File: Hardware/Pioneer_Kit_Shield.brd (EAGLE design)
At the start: 53.3 x 59.7 mm, 38 parts, among them U1 USD-SOCKETNEW, U2 ARDUINO_UNO_R3_SHIELDNOLABELS, U3 HEX_CONVERTER, U4 PCA9306, U5 3.3V

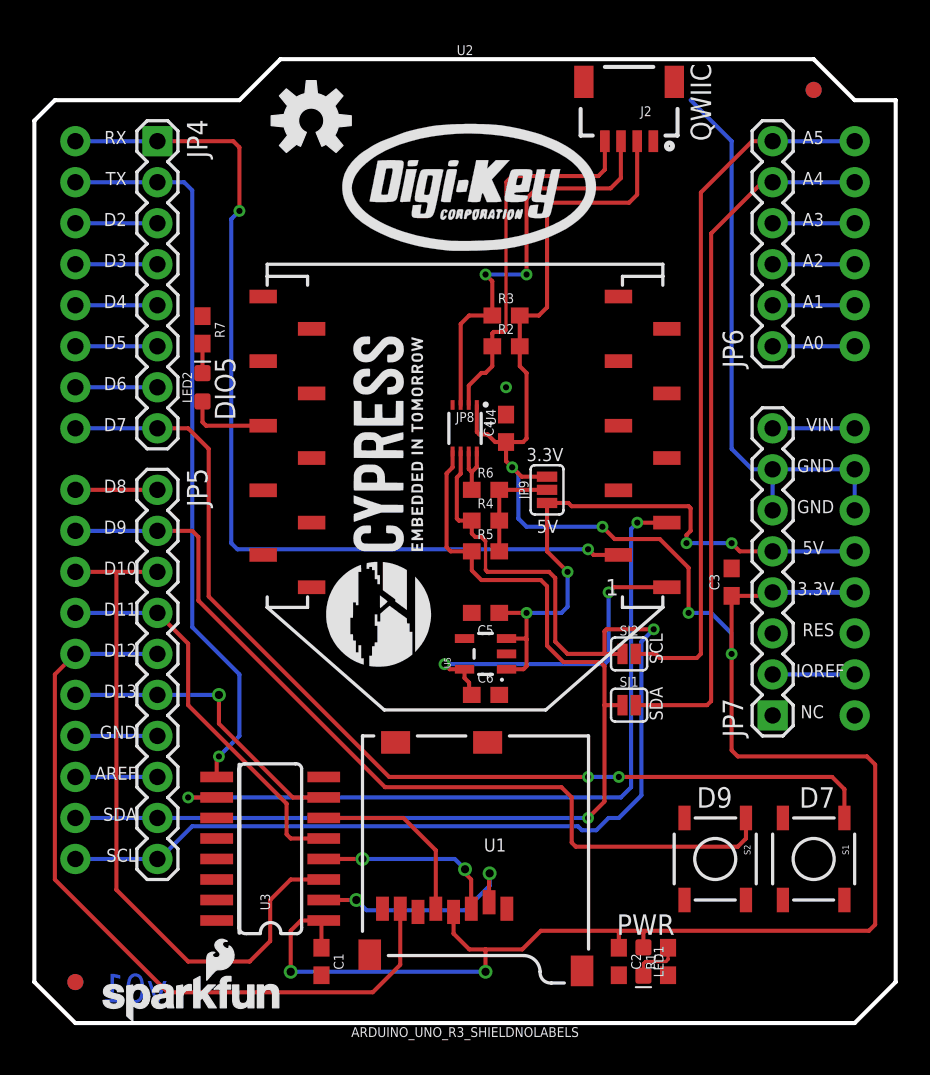
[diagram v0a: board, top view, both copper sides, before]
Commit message: Final version before review
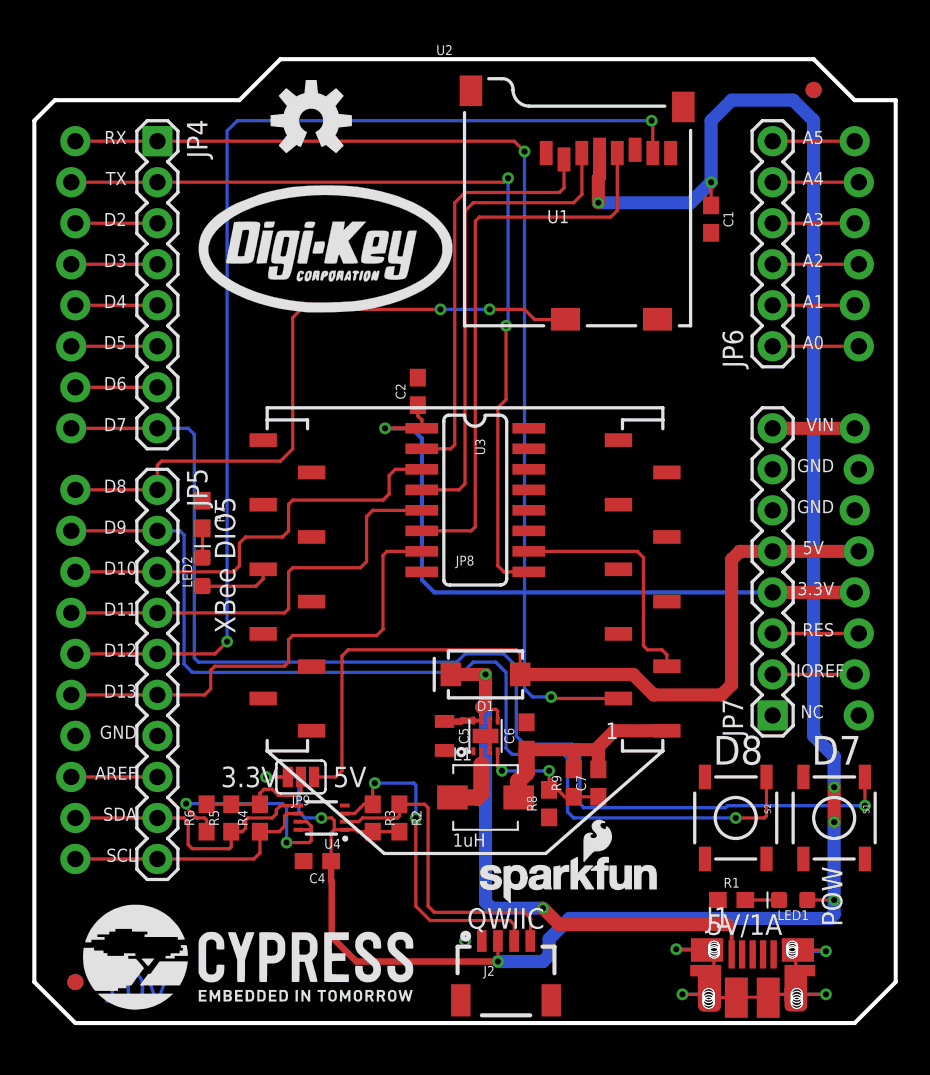
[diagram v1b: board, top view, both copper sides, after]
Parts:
- removed C3: 10uF, SparkFun-Capacitors:0603
- removed SJ1, SJ2: JUMPER-SMT_2_NC_PASTE_SILK, SparkFun-Jumpers:SMT-JUMPER_2_NC_PASTE_SILK
- added C7: 22pF, SparkFun-Capacitors:0603
- added D1: 3A/40V/500mV, SparkFun-DiscreteSemi:SMA-DIODE
- added FRAME2: FRAME-LETTERNO_PACKAGE, SparkFun-Aesthetics:DUMMY
- added J1: AMP FCI 10103594-0001LF, SparkFun-Connectors:USB-MICROB-PTH
- added L1: 1uH, SparkFun-Coils:INDUCTOR-SRP4020
- added R8: 180k, SparkFun-Resistors:0603
- added R9: 820k, SparkFun-Resistors:0603
- C5: value 1.0uF -> 10uF; device SparkFun-Capacitors:0603 -> SparkFun-Capacitors:0805
- C6: value 1.0uF -> 10uF
- U2: value ARDUINO_UNO_R3_SHIELDNOLABELS -> ARDUINO_UNO_R3_SHIELDUNO_R3_SHIELD_NOLABELS_LOCK; device SparkFun-Boards:UNO_R3_SHIELD_NOLABELS -> SparkFun-Boards:UNO_R3_SHIELD_NOLABELS_LOCK
- U5: value 3.3V -> TPS62065; device SparkFun-IC-Power:SOT23-5 -> SparkFun-IC-Power:WSON-8-PAD
- moved C1 51.9 mm to (40.6, 49.8)
- moved J2 50.1 mm to (27.9, 5.08), turned to 0 degrees
- moved C2 37.4 mm to (22.5, 39.1), turned to 90 degrees
- moved U1 32.5 mm to (39.4, 43.2), turned to 0 degrees
- moved R3 32.2 mm to (19.7, 12.7), turned to 270 degrees
- moved R2 29.9 mm to (21.3, 12.7), turned to 270 degrees
- moved C4 29.2 mm to (16.3, 10.0), turned to 180 degrees
- moved R6 26.7 mm to (9.40, 12.7), turned to 90 degrees
- moved U4 25.7 mm to (16.5, 12.7), turned to 90 degrees
- moved U3 25.0 mm to (26.0, 32.4), turned to 270 degrees
- moved JP1 24.5 mm to (25.9, 7.37)
- moved JP9 23.4 mm to (15.2, 15.2), turned to 180 degrees
- moved R4 23.1 mm to (12.7, 12.7), turned to 90 degrees
- moved R5 22.8 mm to (10.9, 12.7), turned to 90 degrees
- moved R7 11.4 mm to (9.14, 31.5)
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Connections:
- removed net D8: JP5.1, U2.D8
- removed net VDD: C6.1, JP8.1, U5.5
- new net !CD: JP5.1, U1.CD2, U2.D8
- new net N$20: C5.1, D1.C, J1.VBUS, U5.5, U5.7, U5.8
- new net N$31: C7.1, R8.2, R9.1, U5.4
- new net N$32: L1.P$1, U5.2
- new net SHIELD: J1.P$1, J1.P$10, J1.P$12, J1.P$2, J1.P$3, J1.P$4, J1.P$6, J1.P$8, J1.SHEILD2, J1.SHIELD, J1.SHIELD3, J1.SHIELD4
- new net VCC: C6.1, C7.2, JP8.1, L1.P$2, R9.2
- net 3.3V: no longer C3.1
- net 5V: now also D1.A; no longer C5.1, U5.1, U5.3
- net A4: no longer SJ1.2
- net A5: no longer SJ2.2
- net GND: now also J1.GND, R8.1, U5.1, U5.3, U5.6, U5.PAD; no longer C3.2, U1.CD1, U1.CD2, U5.2
- net RES: now also U2.RES
- net SCL: no longer SJ2.1
- net SDA: no longer SJ1.1
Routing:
- net SCL: track 73.8 -> 16.1 mm, vias 1 -> 0
- net SDA: track 64.5 -> 17.5 mm, vias 1 -> 0
- net N$20: track 0.00 -> 41.6 mm, vias 0 -> 2
- net !CD: track 0.00 -> 40.9 mm, vias 0 -> 2
- net GND: track 41.2 -> 2.11 mm
- net A4: track 43.9 -> 5.08 mm
- net A5: track 43.7 -> 5.08 mm
- net TX_LV: track 47.8 -> 15.1 mm, vias 2 -> 0
- net 3.3V: track 143.9 -> 173.7 mm, vias 6 -> 9
- net SHIELD: track 0.00 -> 28.0 mm, vias 0 -> 4
- net N$4: track 11.4 -> 35.0 mm
- net MISO: track 48.0 -> 69.9 mm, vias 0 -> 2
- net VDD: track 21.3 -> 0.00 mm, vias 2 -> 0
- net N$2: track 11.6 -> 30.0 mm, vias 2 -> 0
- net !CS: track 43.0 -> 26.5 mm
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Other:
- board text added: "5V/1A"
- board text added: "POW"
- board text added: "XBee DIO5"
- board text removed: "DIO5"
- board text removed: "Original uSD Shield design by R Owens and T Klopfenstein"
- board text removed: "PWR"
